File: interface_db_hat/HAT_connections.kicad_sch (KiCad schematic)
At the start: 12 parts, among them J1 GPIO, J5 Conn_01x04_Pin, U6 MCP23008-xSO

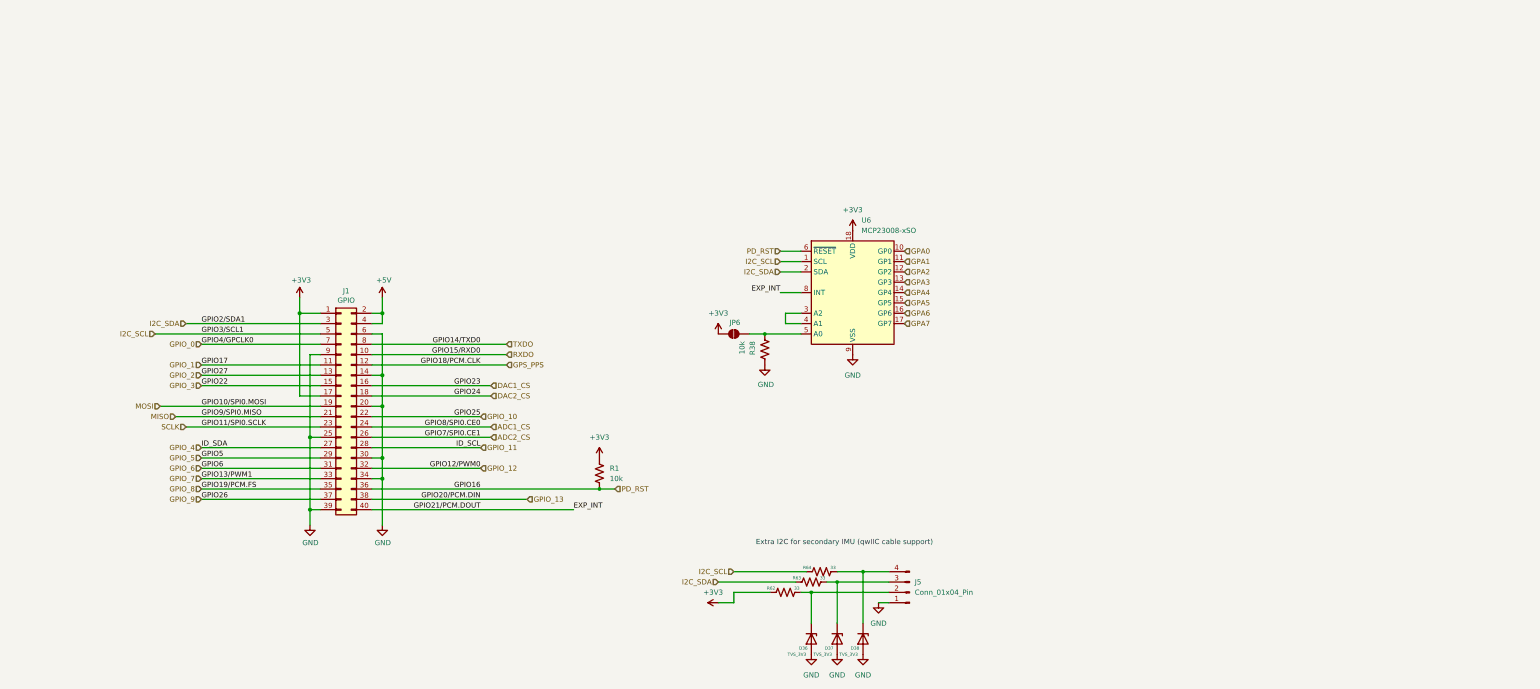
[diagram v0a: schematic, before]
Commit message: lol
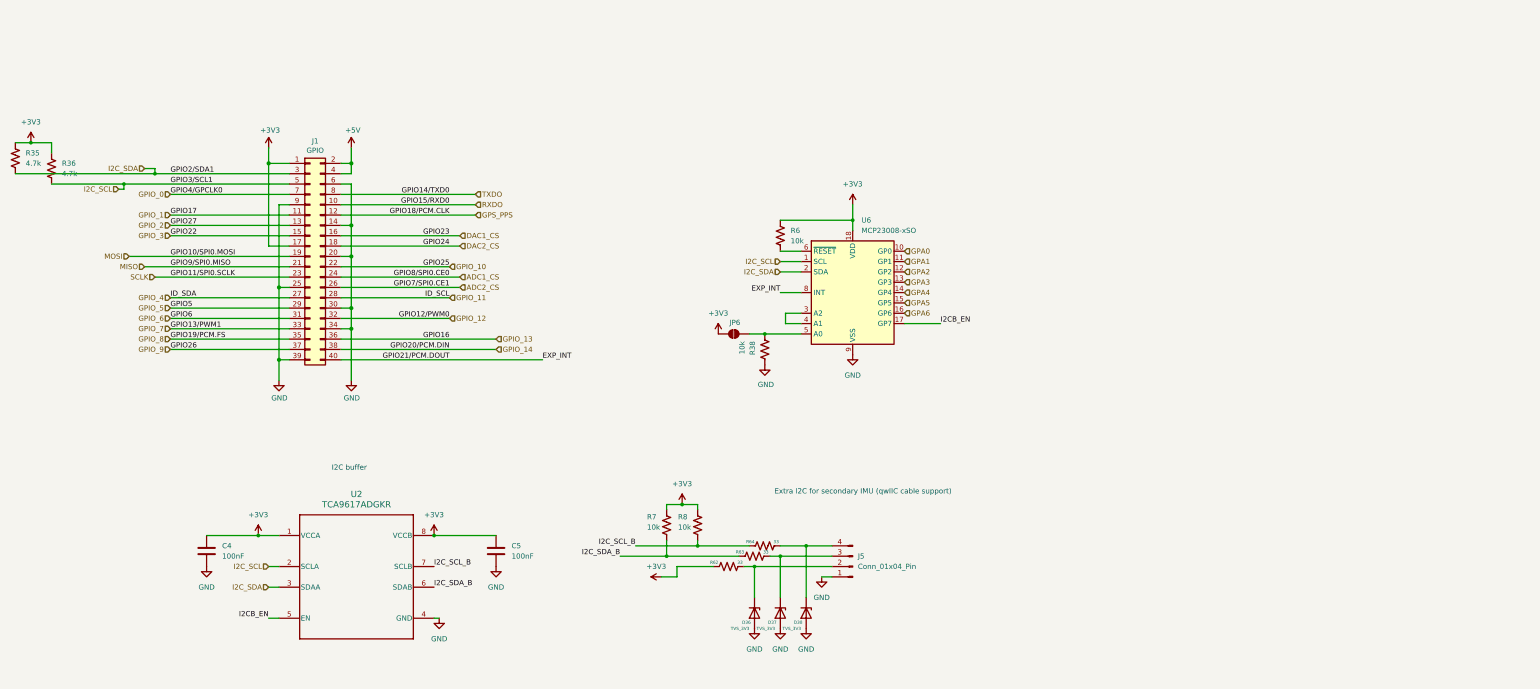
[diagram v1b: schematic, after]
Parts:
- removed R1: 10k, Resistor_SMD:R_0603_1608Metric_Pad0.98x0.95mm_HandSolder, symbol Device:R_US
- added C4, C5: 100nF, symbol Device:C
- added R35, R36: 4.7k, Resistor_SMD:R_0603_1608Metric_Pad0.98x0.95mm_HandSolder, symbol Device:R_US
- added R6, R7, R8: 10k, Resistor_SMD:R_0603_1608Metric_Pad0.98x0.95mm_HandSolder, symbol Device:R_US
- added U2: TCA9617ADGKR, TCA9617:DGK0008A, symbol TCA9617:TCA9617ADGKR
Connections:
- net +3V3: now also C4.1, C5.1, R35.1, R36.1, R6.1, R7.1, R8.1, U2.1 (VCCA), U2.8 (VCCB)
- net GND: now also C4.2, C5.2, U2.4 (GND)
- net GPIO_13: now also J1.36 (Pin_36); no longer J1.38 (Pin_38)
- net I2C_SCL: now also R36.2, U2.2 (SCLA); no longer R64.1
- net I2C_SDA: now also R35.2, U2.3 (SDAA); no longer R63.1
- net GPA7 renamed I2CB_EN
- net I2CB_EN: now also U2.5 (EN)
- net PD_RST: no longer names the net of U6.6 (~{RESET})
- net PD_RST: now also R6.2; no longer J1.36 (Pin_36)
- new net GPIO_14: J1.38 (Pin_38)
- new net I2C_SCL_B: R64.1, R8.2, U2.7 (SCLB)
- new net I2C_SDA_B: R63.1, R7.2, U2.6 (SDAB)
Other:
- note added: "I2C buffer"
- moved on the sheet: D36, D37, D38, J1, J5, R62, R63, R64

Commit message: UPDATE
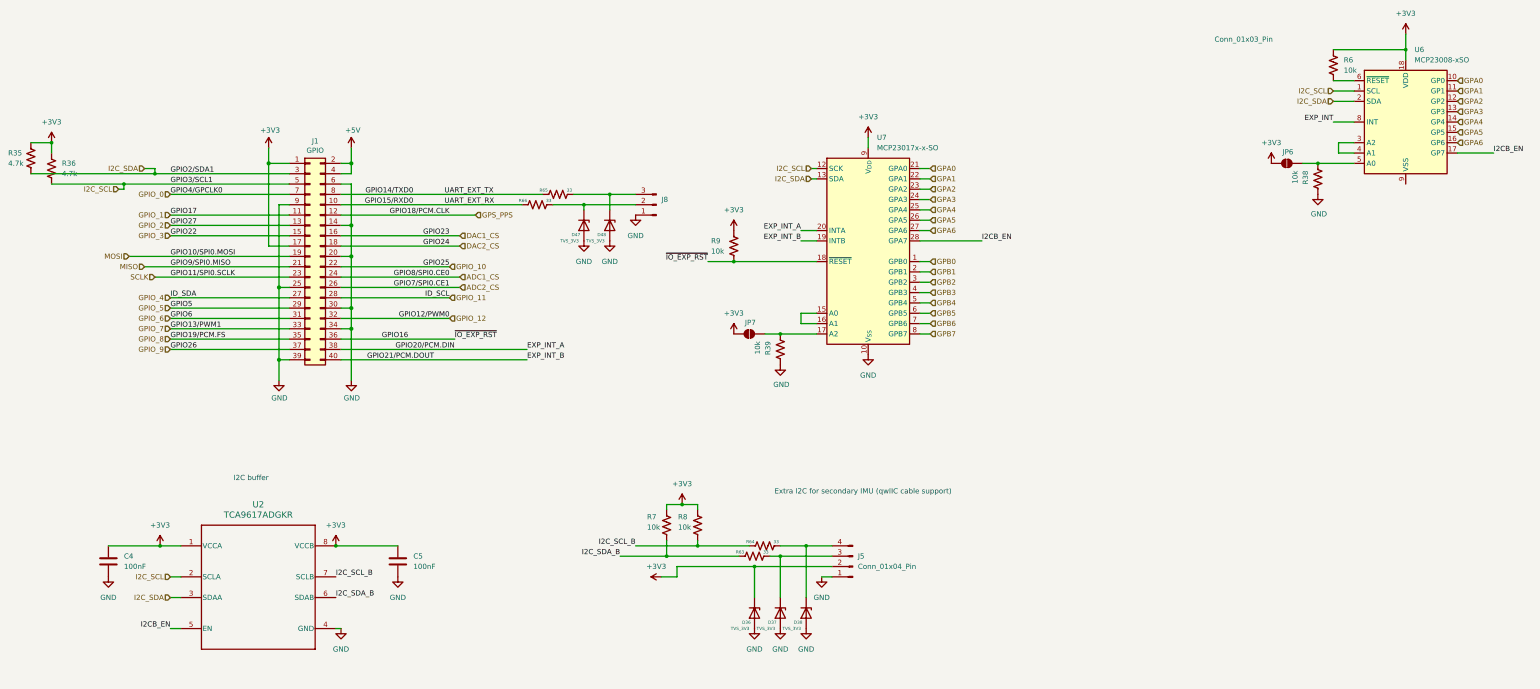
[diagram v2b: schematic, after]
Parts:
- removed R62: 33, Resistor_SMD:R_0603_1608Metric_Pad0.98x0.95mm_HandSolder, symbol Device:R_US
- added D47, D48: TVS_3V3, Diode_SMD:D_0402_1005Metric_Pad0.77x0.64mm_HandSolder, symbol Device:D_Zener
- added J8: Conn_01x03_Pin, Connector_PinHeader_2.54mm:PinHeader_1x03_P2.54mm_Horizontal, symbol Connector:Conn_01x03_Pin
- added JP7: SolderJumper_2_Open, Jumper:SolderJumper-2_P1.3mm_Open_TrianglePad1.0x1.5mm, symbol Jumper:SolderJumper_2_Open
- added R39, R9: 10k, Resistor_SMD:R_0603_1608Metric_Pad0.98x0.95mm_HandSolder, symbol Device:R_US
- added R65, R66: 33, Resistor_SMD:R_0603_1608Metric_Pad0.98x0.95mm_HandSolder, symbol Device:R_US
- added U7: MCP23017x-x-SO, Package_SO:SOIC-28W_7.5x17.9mm_P1.27mm, symbol Interface_Expansion:MCP23017x-x-SO
- C4, C5: footprint (none) -> Capacitor_SMD:C_0603_1608Metric_Pad1.08x0.95mm_HandSolder
- D36, D37, D38: footprint Diode_SMD:D_0603_1608Metric_Pad1.05x0.95mm_HandSolder -> Diode_SMD:D_0402_1005Metric_Pad0.77x0.64mm_HandSolder
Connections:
- net +3V3: now also D36.1 (K), J5.2 (Pin_2), JP7.2 (B), R9.2, U7.9 (V_{DD})
- net EXP_INT: no longer J1.40 (Pin_40)
- net GND: now also D47.2 (A), D48.2 (A), J8.1 (Pin_1), R39.2, U7.10 (V_{SS}); no longer U6.9 (VSS)
- net GPA0: now also U7.21 (GPA0)
- net GPA1: now also U7.22 (GPA1)
- net GPA2: now also U7.23 (GPA2)
- net GPA3: now also U7.24 (GPA3)
- net GPA4: now also U7.25 (GPA4)
- net GPA5: now also U7.26 (GPA5)
- net GPA6: now also U7.27 (GPA6)
- net I2CB_EN: now also U7.28 (GPA7)
- net I2C_SCL: now also U7.12 (SCK)
- net I2C_SDA: now also U7.13 (SDA)
- net GPIO_13 renamed GPIO16
- net GPIO16: now also R9.1, U7.18 (~{RESET})
- net GPIO_14 renamed EXP_INT_A
- net EXP_INT_A: now also U7.20 (INTA)
- net RXDO renamed GPIO15/RXD0
- net GPIO15/RXD0: now also R66.1
- net TXDO renamed GPIO14/TXD0
- net GPIO14/TXD0: now also R65.1
- new net: D48.1 (K), J8.3 (Pin_3), R65.2
- new net: D47.1 (K), J8.2 (Pin_2), R66.2
- new net: U7.15 (A0), U7.16 (A1)
- new net: JP7.1 (A), R39.1, U7.17 (A2)
- new net EXP_INT_B: J1.40 (Pin_40), U7.19 (INTB)
- new net GPB0: U7.1 (GPB0)
- new net GPB1: U7.2 (GPB1)
- new net GPB2: U7.3 (GPB2)
- new net GPB3: U7.4 (GPB3)
- new net GPB4: U7.5 (GPB4)
- new net GPB5: U7.6 (GPB5)
- new net GPB6: U7.7 (GPB6)
- new net GPB7: U7.8 (GPB7)
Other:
- moved on the sheet: C4, C5, JP6, R35, R38, R6, U2, U6
